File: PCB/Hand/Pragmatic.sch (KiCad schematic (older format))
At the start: 80 parts, among them J1 Conn_02x08_Odd_Even, J2 Conn_01x04, SW1 SW_Push, SW10 SW_Push, SW11 SW_Push, SW12 SW_Push, SW13 SW_Push, SW14 Q, SW15 W, SW16 E, SW17 R, SW18 T, SW19 SW_Push, SW2 SW_Push, SW20 A, SW21 S, SW22 D, SW23 F, SW24 G, SW25 SW_Push, SW26 Z, SW27 X, SW28 C, SW29 V, SW3 SW_Push, SW30 B, SW31 SW_Push, SW32 SW_Push, SW33 SW_Push, SW34 SW_Push, SW35 SW_Push, SW36 SW_Push, SW4 SW_Push, SW5 SW_Push, SW6 SW_Push, SW7 SW_Push, SW8 SW_Push, SW9 SW_Push

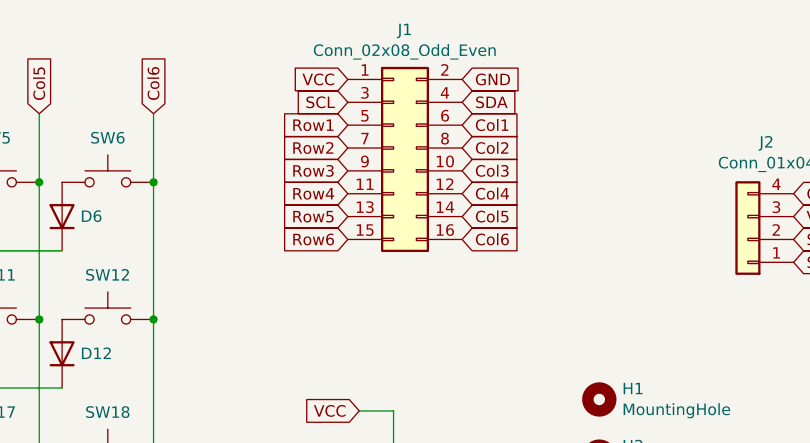
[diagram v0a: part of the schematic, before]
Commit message: controller done
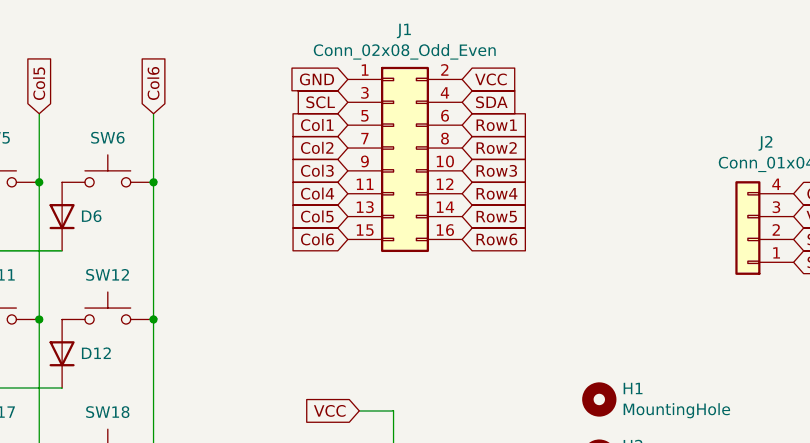
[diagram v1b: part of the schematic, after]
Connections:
- net +5V: now also J1.2 (Pin_2); no longer J1.1 (Pin_1)
- net Col1: now also J1.5 (Pin_5); no longer J1.6 (Pin_6)
- net Col2: now also J1.7 (Pin_7); no longer J1.8 (Pin_8)
- net Col3: now also J1.9 (Pin_9); no longer J1.10 (Pin_10)
- net Col4: now also J1.11 (Pin_11); no longer J1.12 (Pin_12)
- net Col5: now also J1.13 (Pin_13); no longer J1.14 (Pin_14)
- net Col6: now also J1.15 (Pin_15); no longer J1.16 (Pin_16)
- net GND: now also J1.1 (Pin_1); no longer J1.2 (Pin_2)
- net Row1: now also J1.6 (Pin_6); no longer J1.5 (Pin_5)
- net Row2: now also J1.8 (Pin_8); no longer J1.7 (Pin_7)
- net Row3: now also J1.10 (Pin_10); no longer J1.9 (Pin_9)
- net Row4: now also J1.12 (Pin_12); no longer J1.11 (Pin_11)
- net Row5: now also J1.14 (Pin_14); no longer J1.13 (Pin_13)
- net Row6: now also J1.16 (Pin_16); no longer J1.15 (Pin_15)
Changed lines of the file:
@@
 	10550 4050 10150 4050
 Connection ~ 10150 4050
+Text GLabel 6250 2550 2    50   Input ~ 0
+VCC
 Text GLabel 5750 2550 0    50   Input ~ 0
-VCC
-Text GLabel 6250 2550 2    50   Input ~ 0
 GND
 Text GLabel 6250 2650 2    50   Input ~ 0
@@
 Text GLabel 5750 2650 0    50   Input ~ 0
 SCL
-Text GLabel 5750 2750 0    50   Input ~ 0
+Text GLabel 6250 2750 2    50   Input ~ 0
 Row1
+Text GLabel 6250 2850 2    50   Input ~ 0
+Row2
+Text GLabel 6250 2950 2    50   Input ~ 0
+Row3
+Text GLabel 6250 3050 2    50   Input ~ 0
+Row4
+Text GLabel 6250 3150 2    50   Input ~ 0
+Row5
+Text GLabel 6250 3250 2    50   Input ~ 0
+Row6
 Text GLabel 5750 2850 0    50   Input ~ 0
-Row2
+Col2
 Text GLabel 5750 2950 0    50   Input ~ 0
-Row3
+Col3
 Text GLabel 5750 3050 0    50   Input ~ 0
-Row4
-Text GLabel 5750 3150 0    50   Input ~ 0
-Row5
+Col4
 Text GLabel 5750 3250 0    50   Input ~ 0
-Row6
-Text GLabel 6250 2750 2    50   Input ~ 0
-Col1
-Text GLabel 6250 2850 2    50   Input ~ 0
-Col2
-Text GLabel 6250 2950 2    50   Input ~ 0
-Col3
-Text GLabel 6250 3050 2    50   Input ~ 0
-Col4
-Text GLabel 6250 3150 2    50   Input ~ 0
-Col5
-Text GLabel 6250 3250 2    50   Input ~ 0
 Col6
 Text GLabel 7700 3050 2    50   Input ~ 0
@@
 Text GLabel 7700 3150 2    50   Input ~ 0
 VCC
-$Comp
-L Connector_Generic:Conn_02x08_Odd_Even J1
-U 1 1 6194905D
-P 5950 2850
-F 0 "J1" H 6000 3367 50  0000 C CNN
-F 1 "Conn_02x08_Odd_Even" H 6000 3276 50  0000 C CNN
-F 2 "Pragmatic:IDC-Header_2x08_P2.54mm_Vertical_Mirrored" H 5950 2850 50  0001 C CNN
-F 3 "~" H 5950 2850 50  0001 C CNN
-F 4 "C3406" H 5950 2850 50  0001 C CNN "LCSC"
-	1    5950 2850
-	1    0    0    -1
-$EndComp
 $Comp
 L Connector_Generic:Conn_01x04 J2
@@
 	1    0    0    -1
 $EndComp
+$Comp
+L Connector_Generic:Conn_02x08_Odd_Even J1
+U 1 1 6194905D
+P 5950 2850
+F 0 "J1" H 6000 3367 50  0000 C CNN
+F 1 "Conn_02x08_Odd_Even" H 6000 3276 50  0000 C CNN
+F 2 "Pragmatic:IDC-Header_2x08_P2.54mm_Vertical_Mirrored" H 5950 2850 50  0001 C CNN
+F 3 "~" H 5950 2850 50  0001 C CNN
+F 4 "C3406" H 5950 2850 50  0001 C CNN "LCSC"
+	1    5950 2850
+	1    0    0    -1
+$EndComp
+Text GLabel 5750 2750 0    50   Input ~ 0
+Col1
+Text GLabel 5750 3150 0    50   Input ~ 0
+Col5
 $EndSCHEMATC
